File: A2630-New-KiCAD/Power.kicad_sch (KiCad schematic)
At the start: 25 parts, among them U204 74HCT04, U300 74HCT05, U307 74HCT04, U507 74HCT74, U606 74HCT244, U800 LM1117-3.3

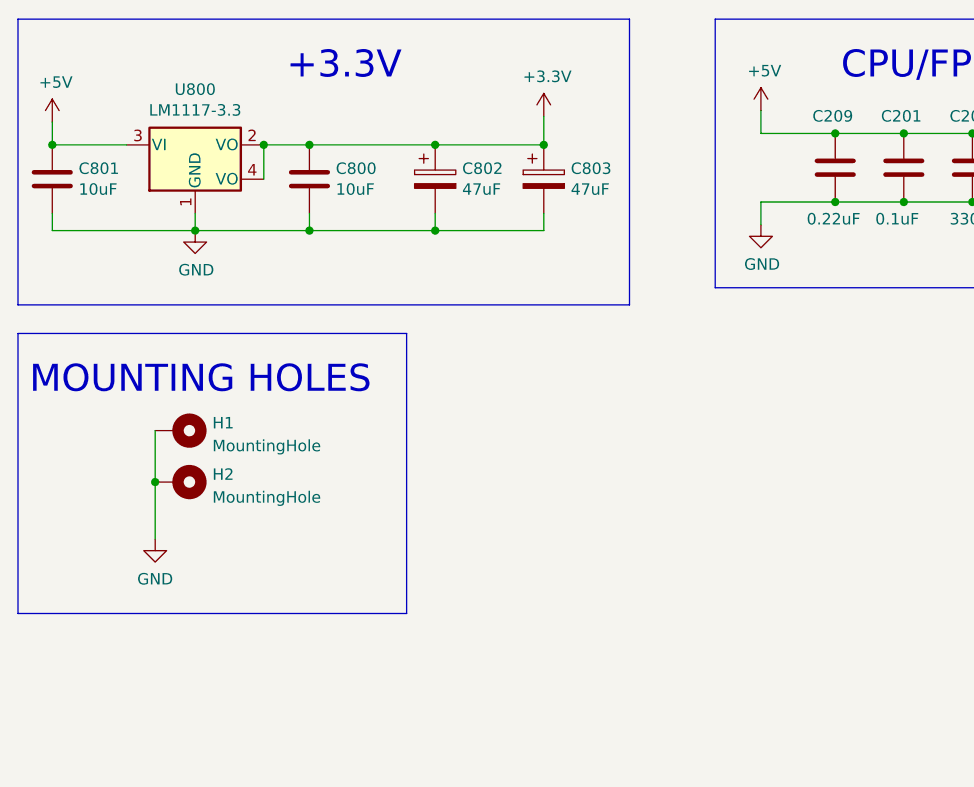
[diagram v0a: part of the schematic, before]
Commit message: Add files via upload
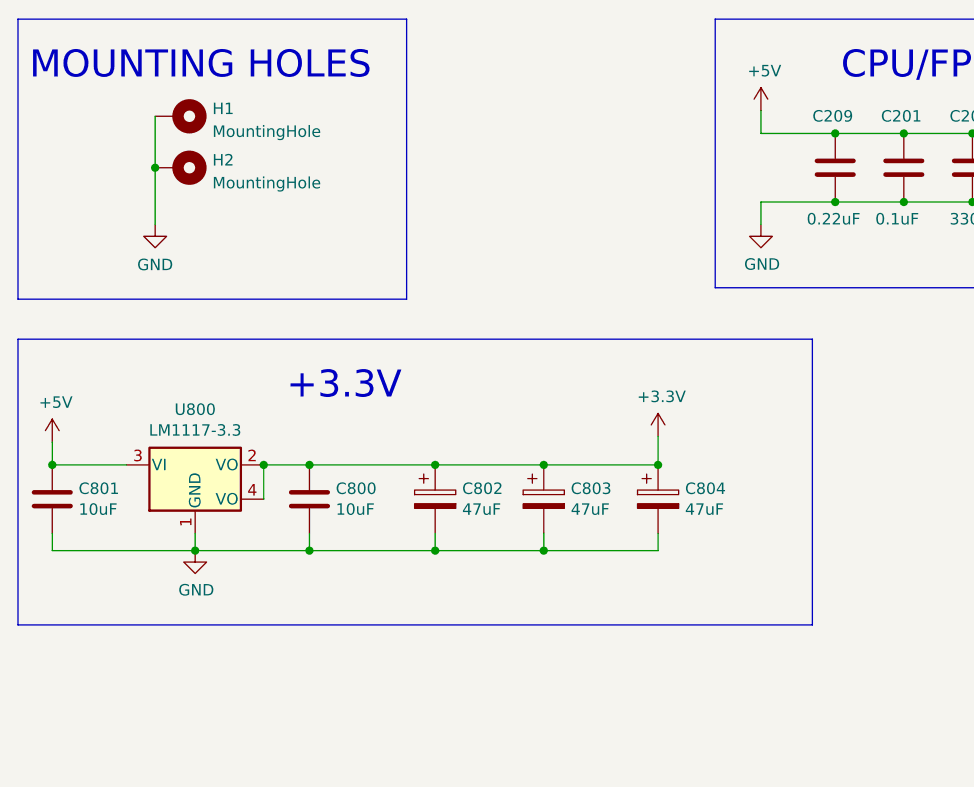
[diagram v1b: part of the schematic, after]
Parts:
- added C804: 47uF, Capacitor_THT:CP_Radial_D5.0mm_P2.00mm, symbol Device:CP
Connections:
- net +3V3: now also C804.1
- net GND: now also C804.2
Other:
- moved on the sheet: C800, C801, C802, C803, H1, H2, U800
